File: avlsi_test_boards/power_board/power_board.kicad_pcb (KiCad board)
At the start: 6 copper layers, 100 x 100 mm, 100 parts, among them J1 PJ-102AH, J2 PJ-102AH, U1 TLV1117LV18DCYR, U11 TLV75709PDBV, U12 SN74LVC16T245DLR, U13 SN74LVC16T245DLR, U14 SN74LVC16T245DLR, U15 SN74LVC16T245DLR, U16 SN74LVC16T245DLR, U17 SN74LVC16T245DLR, U2 TLV1117LV25DCYR, U3 TLV1117LV33DCYR, U4 DS04-254-2-04BK-SMT, U5 74HC4051D_653, U6 TLV1117LV18DCYR, U7 TLV75709PDBV, U8 TLV1117LV25DCYR, U9 TLV1117LV33DCYR

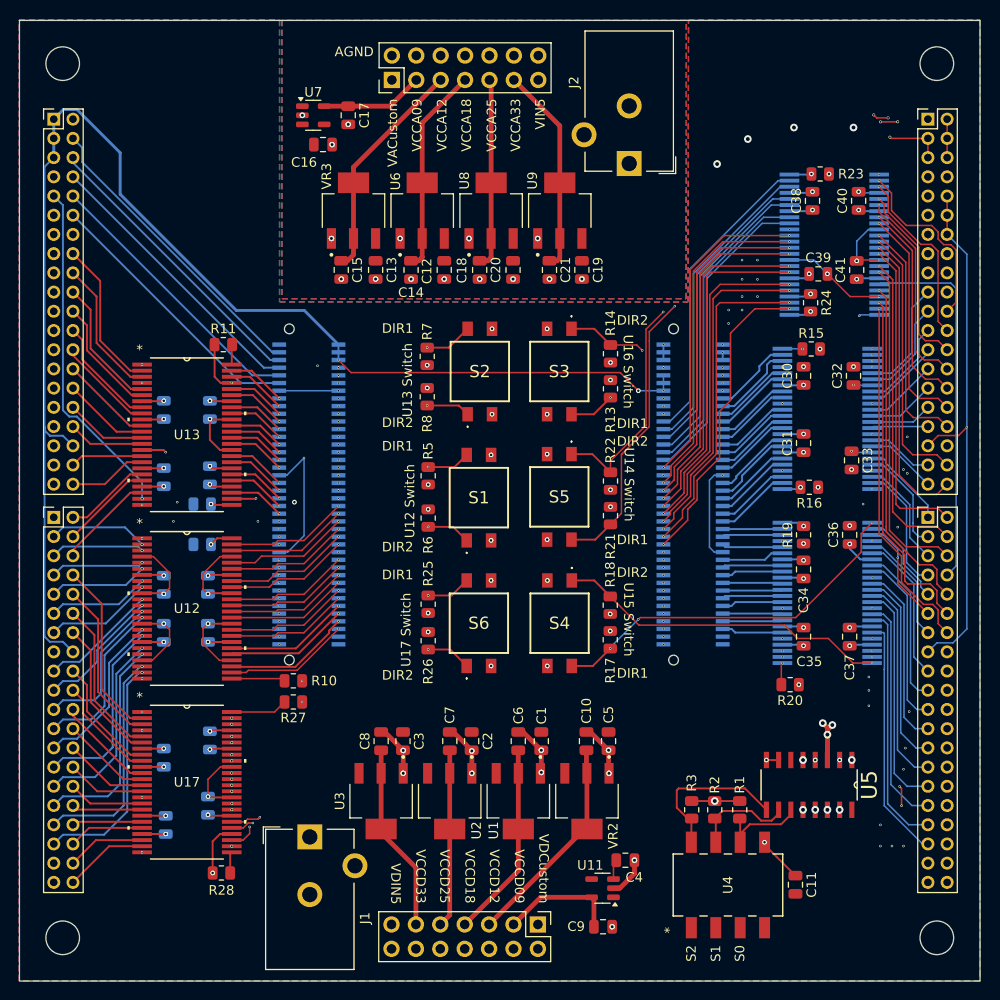
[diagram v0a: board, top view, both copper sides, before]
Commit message: Update schematic
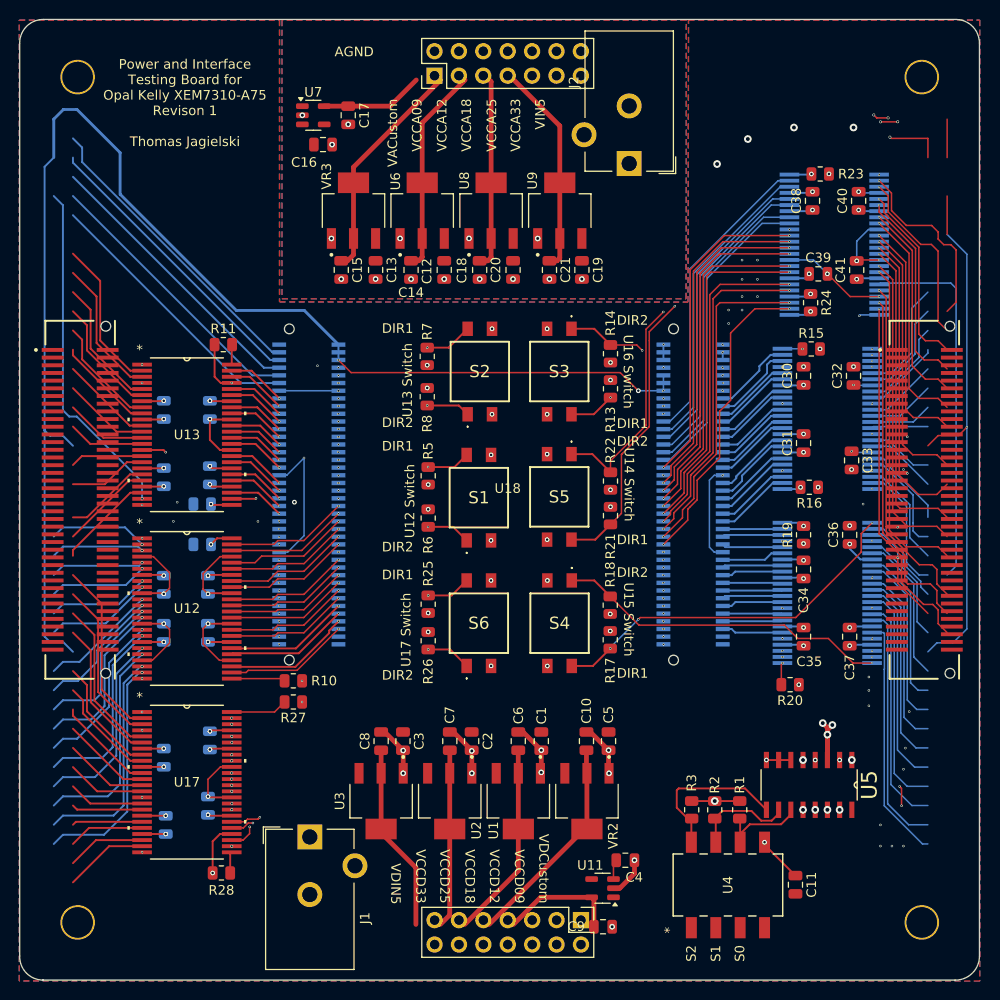
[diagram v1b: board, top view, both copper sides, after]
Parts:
- U18: footprint avlsi_preferred_parts:avlsi_power_board_opal_kelly -> avlsi_preferred_parts:power_board
- moved U18 3.06 mm to (151.0, 74.7)
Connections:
- net ADGND renamed AGND
- U18 pad 177: VCCD09 -> (no net)
- U18 pad 178: DGND -> (no net)
- U18 pad 179: VCCD12 -> VCCD09
- U18 pad 181: VCCD18 -> VCCD12
- U18 pad 183: VCCD25 -> VCCD18
- U18 pad 185: VCCD33 -> VCCD25
- U18 pad 187: DVIN5 -> VCCD33
- U5 pad 6: DVIN5 -> DGND
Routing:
- net FPGA_33VDD: track 272.7 -> 220.9 mm, vias 7 -> 6
- net MC1_23_PIN: track 18.5 -> 70.4 mm, vias 1 -> 2
- net DGND: track 155.3 -> 156.5 mm
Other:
- board size 100 x 100 mm -> 99.9 x 100 mm
- board text added: "Power and Interface Testing Board for Opal Kelly XEM7310-A75 Revison 1 Thomas Jagielski"
